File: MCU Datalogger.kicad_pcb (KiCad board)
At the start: 4 copper layers, 50.8 x 30.5 mm, 29 parts, among them J1 Conn_01x04_Male, J2 Conn_01x09_Male, J3 Conn_01x04_Male, J4 Conn_02x03_Odd_Even, U1 24LC1025, U2 DS1337S+, U3 24LC1025, U4 ATMEGA328-AU, Y1 32.768KHz, Y2 16MHz

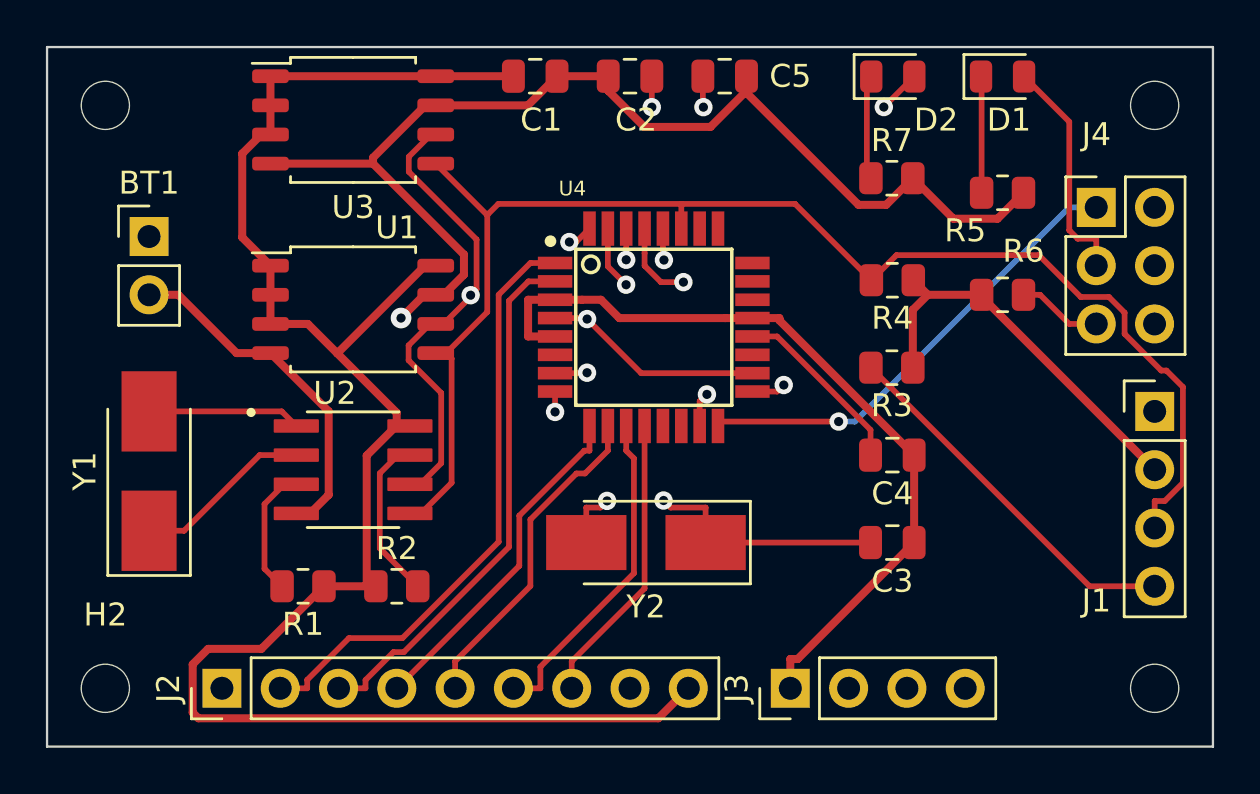
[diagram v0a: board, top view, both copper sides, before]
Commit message: error
git commit -amerror
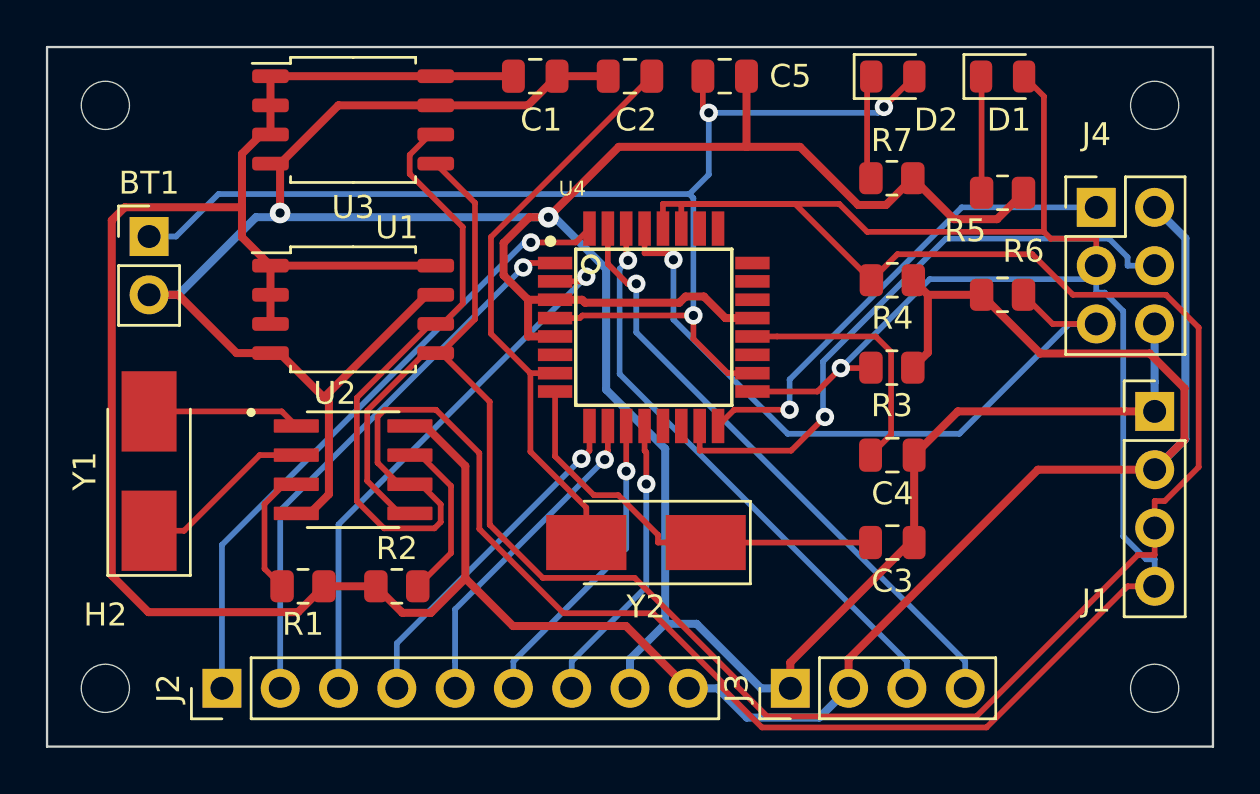
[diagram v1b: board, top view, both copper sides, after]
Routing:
- net /SDA: track 61.8 -> 100.9 mm
- net /SCK: track 98.3 -> 137.3 mm, vias 3 -> 1
- net /Vcc: track 133.3 -> 148.5 mm
- net /RESET: track 26.0 -> 31.2 mm
- net Net-(U4-Pad18): track 51.3 -> 55.2 mm
- net /TX: track 30.1 -> 26.7 mm
- net Net-(U4-Pad20): track 7.93 -> 11.2 mm
- net /MOSI: track 23.8 -> 27.0 mm
- net /D3: track 26.2 -> 24.2 mm, vias 0 -> 1
- net Net-(C2-Pad2): track 24.1 -> 26.0 mm, vias 3 -> 0
- net GND: track 165.1 -> 163.5 mm, vias 1 -> 2
- net /D2: track 26.8 -> 28.0 mm
- net /D7: track 14.4 -> 13.5 mm, vias 0 -> 1
- net /MISO: track 20.4 -> 21.2 mm
- net /D4: track 23.3 -> 23.8 mm, vias 0 -> 1
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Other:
- copper layers 4 -> 2

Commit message: routing
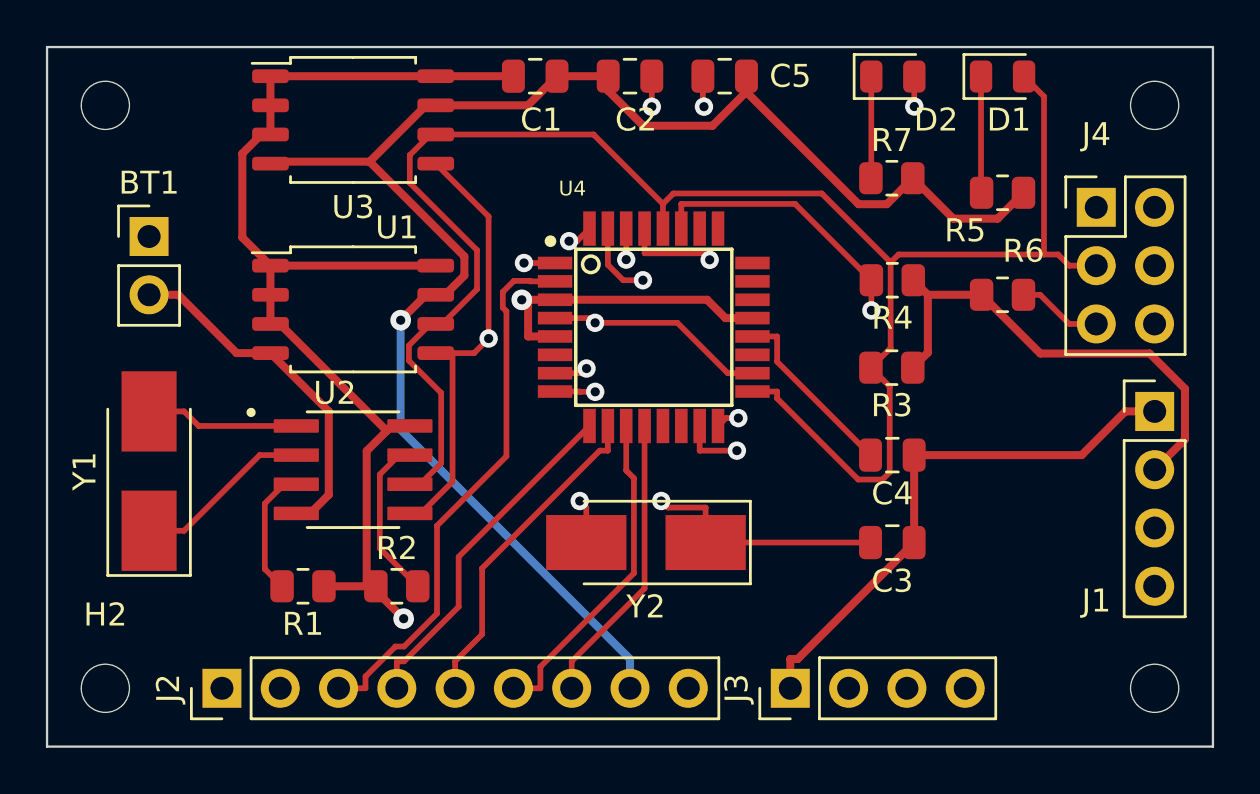
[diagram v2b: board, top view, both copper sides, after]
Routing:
- net /SCK: track 137.3 -> 94.6 mm, vias 1 -> 0
- net /SDA: track 100.9 -> 68.5 mm, vias 0 -> 2
- net /Vcc: track 148.5 -> 122.0 mm, vias 0 -> 1
- net GND: track 163.5 -> 152.3 mm
- net /RESET: track 31.2 -> 25.7 mm
- net Net-(U4-Pad20): track 11.2 -> 7.93 mm
- net Net-(C2-Pad2): track 26.0 -> 23.6 mm, vias 0 -> 3
- net Net-(U4-Pad18): track 55.2 -> 52.8 mm
- net /MOSI: track 27.0 -> 25.4 mm
- net /TX: track 26.7 -> 27.7 mm
- net /D7: track 13.5 -> 14.4 mm, vias 1 -> 0
- net /MISO: track 21.2 -> 20.4 mm
- net /D6: track 14.2 -> 14.4 mm, vias 1 -> 0
- net /D5: track 14.9 -> 15.1 mm, vias 1 -> 0
- net Net-(Y2-Pad1): track 18.3 -> 18.5 mm, vias 0 -> 2
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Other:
- copper layers 2 -> 4
